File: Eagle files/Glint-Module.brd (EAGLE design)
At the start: 50.8 x 25.4 mm, 17 parts

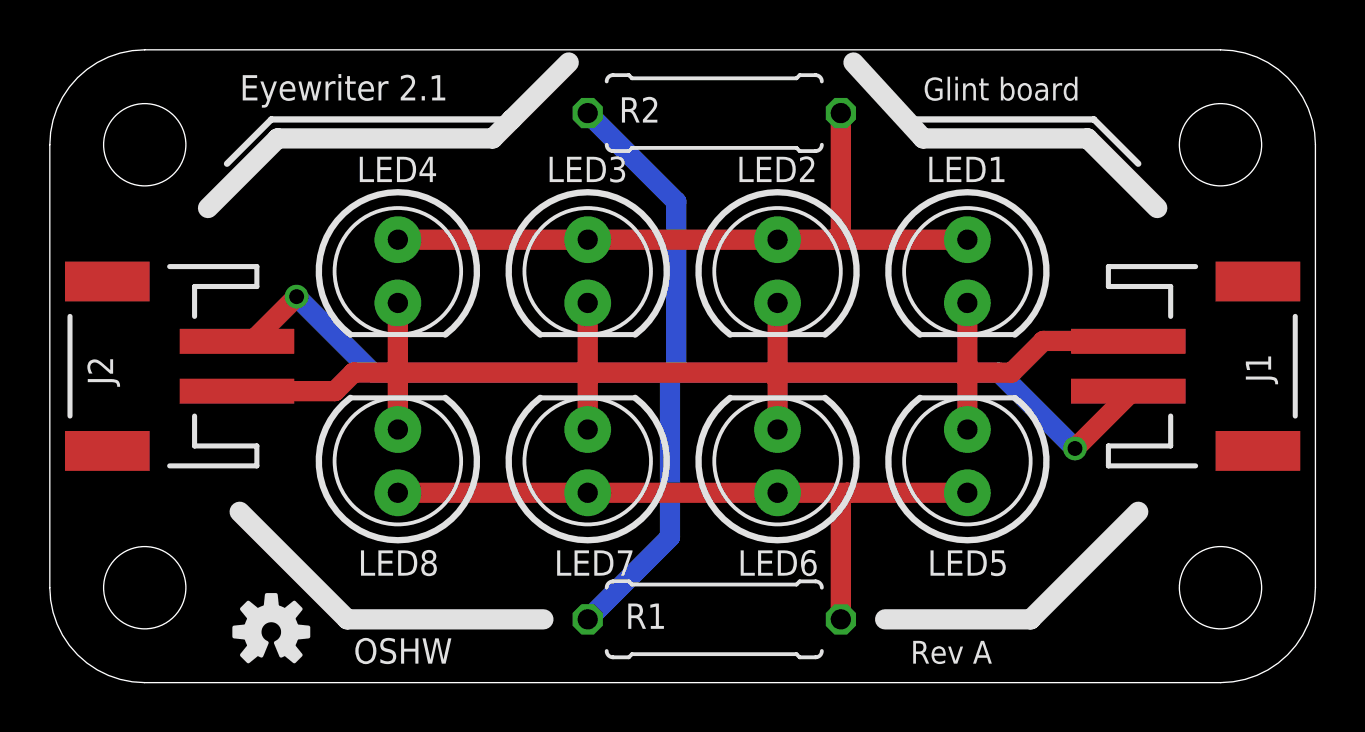
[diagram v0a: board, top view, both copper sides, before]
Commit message: Updated Eagle files + BOMs
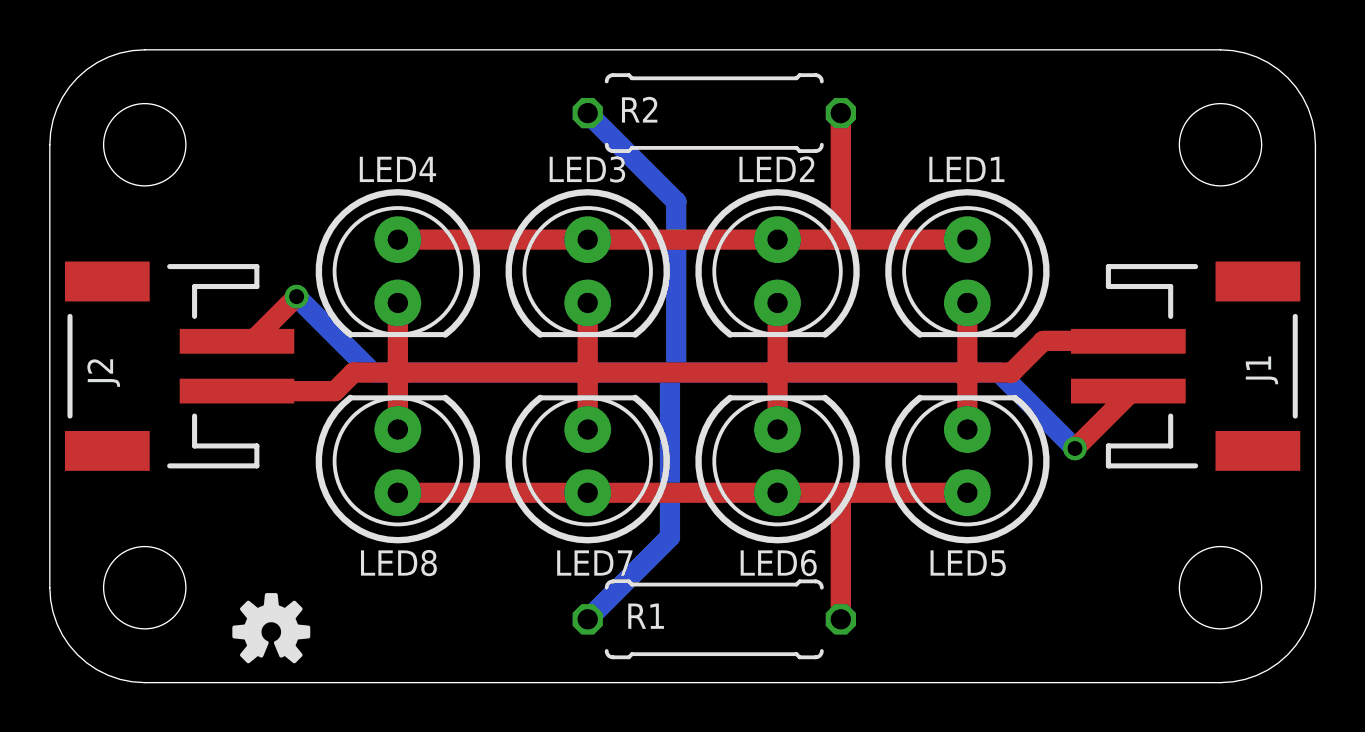
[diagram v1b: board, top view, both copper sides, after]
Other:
- board text added: "Designed by Jason Webb (http://jason-webb.info)"
- board text removed: "Designed by Jason Webb - http://jason-webb.info"
- board text removed: "Rev A"
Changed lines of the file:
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@@
 <layer number="20" name="Dimension" color="15" fill="1" visible="yes" active="yes"/>
 <layer number="21" name="tPlace" color="7" fill="1" visible="yes" active="yes"/>
-<layer number="22" name="bPlace" color="7" fill="1" visible="no" active="yes"/>
+<layer number="22" name="bPlace" color="7" fill="1" visible="yes" active="yes"/>
 <layer number="23" name="tOrigins" color="15" fill="1" visible="yes" active="yes"/>
-<layer number="24" name="bOrigins" color="15" fill="1" visible="no" active="yes"/>
+<layer number="24" name="bOrigins" color="15" fill="1" visible="yes" active="yes"/>
 <layer number="25" name="tNames" color="7" fill="1" visible="yes" active="yes"/>
-<layer number="26" name="bNames" color="7" fill="1" visible="no" active="yes"/>
+<layer number="26" name="bNames" color="7" fill="1" visible="yes" active="yes"/>
 <layer number="27" name="tValues" color="7" fill="1" visible="yes" active="yes"/>
-<layer number="28" name="bValues" color="7" fill="1" visible="no" active="yes"/>
+<layer number="28" name="bValues" color="7" fill="1" visible="yes" active="yes"/>
 <layer number="29" name="tStop" color="7" fill="3" visible="no" active="yes"/>
 <layer number="30" name="bStop" color="7" fill="6" visible="no" active="yes"/>
@@
 <layer number="37" name="tTest" color="7" fill="1" visible="no" active="yes"/>
 <layer number="38" name="bTest" color="7" fill="1" visible="no" active="yes"/>
-<layer number="39" name="tKeepout" color="4" fill="11" visible="no" active="yes"/>
-<layer number="40" name="bKeepout" color="1" fill="11" visible="no" active="yes"/>
-<layer number="41" name="tRestrict" color="4" fill="10" visible="no" active="yes"/>
-<layer number="42" name="bRestrict" color="1" fill="10" visible="no" active="yes"/>
-<layer number="43" name="vRestrict" color="2" fill="10" visible="no" active="yes"/>
+<layer number="39" name="tKeepout" color="4" fill="11" visible="yes" active="yes"/>
+<layer number="40" name="bKeepout" color="1" fill="11" visible="yes" active="yes"/>
+<layer number="41" name="tRestrict" color="4" fill="10" visible="yes" active="yes"/>
+<layer number="42" name="bRestrict" color="1" fill="10" visible="yes" active="yes"/>
+<layer number="43" name="vRestrict" color="2" fill="10" visible="yes" active="yes"/>
 <layer number="44" name="Drills" color="7" fill="1" visible="no" active="yes"/>
 <layer number="45" name="Holes" color="7" fill="1" visible="no" active="yes"/>
 <layer number="46" name="Milling" color="3" fill="1" visible="no" active="yes"/>
 <layer number="47" name="Measures" color="7" fill="1" visible="no" active="yes"/>
-<layer number="48" name="Document" color="7" fill="1" visible="no" active="yes"/>
-<layer number="49" name="Reference" color="7" fill="1" visible="no" active="yes"/>
+<layer number="48" name="Document" color="7" fill="1" visible="yes" active="yes"/>
+<layer number="49" name="Reference" color="7" fill="1" visible="yes" active="yes"/>
 <layer number="50" name="dxf" color="7" fill="1" visible="no" active="no"/>
-<layer number="51" name="tDocu" color="7" fill="1" visible="no" active="yes"/>
+<layer number="51" name="tDocu" color="7" fill="1" visible="yes" active="yes"/>
 <layer number="52" name="bDocu" color="7" fill="1" visible="no" active="yes"/>
 <layer number="53" name="tGND_GNDA" color="7" fill="9" visible="no" active="no"/>
@@
 <layer number="144" name="Drill_legend" color="7" fill="1" visible="no" active="yes"/>
 <layer number="151" name="HeatSink" color="7" fill="1" visible="no" active="yes"/>
-<layer number="199" name="Contour" color="7" fill="1" visible="no" active="yes"/>
+<layer number="199" name="Contour" color="7" fill="1" visible="yes" active="yes"/>
 <layer number="200" name="200bmp" color="1" fill="10" visible="no" active="yes"/>
 <layer number="201" name="201bmp" color="2" fill="10" visible="no" active="yes"/>
@@
 <board>
 <plain>
-<text x="7.62" y="23.368" size="1.016" layer="21" font="vector" ratio="16">Eyewriter 2.1</text>
-<text x="35.052" y="23.368" size="0.9144" layer="21" font="vector" ratio="12">Glint board</text>
-<wire x1="17.78" y1="21.844" x2="18.542" y2="22.606" width="0.8128" layer="21"/>
-<wire x1="18.542" y1="22.606" x2="20.828" y2="24.892" width="0.8128" layer="21"/>
-<wire x1="35.052" y1="21.844" x2="32.258" y2="24.892" width="0.8128" layer="21"/>
-<wire x1="17.78" y1="21.844" x2="9.144" y2="21.844" width="0.8128" layer="21"/>
-<wire x1="9.144" y1="21.844" x2="6.35" y2="19.05" width="0.8128" layer="21"/>
-<wire x1="35.052" y1="21.844" x2="41.656" y2="21.844" width="0.8128" layer="21"/>
-<wire x1="41.656" y1="21.844" x2="44.45" y2="19.05" width="0.8128" layer="21"/>
-<wire x1="34.544" y1="22.606" x2="41.91" y2="22.606" width="0.254" layer="21"/>
-<wire x1="41.91" y1="22.606" x2="43.688" y2="20.828" width="0.254" layer="21"/>
-<wire x1="18.542" y1="22.606" x2="8.89" y2="22.606" width="0.254" layer="21"/>
-<wire x1="8.89" y1="22.606" x2="7.112" y2="20.828" width="0.254" layer="21"/>
-<wire x1="7.62" y1="6.858" x2="11.938" y2="2.54" width="0.8128" layer="21"/>
-<wire x1="11.938" y1="2.54" x2="19.812" y2="2.54" width="0.8128" layer="21"/>
-<wire x1="43.688" y1="6.858" x2="39.37" y2="2.54" width="0.8128" layer="21"/>
-<wire x1="39.37" y1="2.54" x2="33.528" y2="2.54" width="0.8128" layer="21"/>
-<text x="12.192" y="0.762" size="1.016" layer="21" font="vector" ratio="16">OSHW</text>
-<text x="25.4" y="4.572" size="0.889" layer="22" font="vector" ratio="10" rot="MR0" align="center">Designed by Jason Webb - http://jason-webb.info</text>
-<text x="42.164" y="12.192" size="1.27" layer="22" font="vector" ratio="16" rot="MR0">Eyewrtier 2.1</text>
-<text x="21.082" y="12.446" size="1.27" layer="22" font="vector" ratio="16" rot="MR0">Glint board</text>
+<text x="7.62" y="23.368" size="1.016" layer="51" font="vector" ratio="16">Eyewriter 2.1</text>
+<text x="35.052" y="23.368" size="0.9144" layer="51" font="vector" ratio="12">Glint board</text>
+<wire x1="17.78" y1="21.844" x2="18.542" y2="22.606" width="0.8128" layer="51"/>
+<wire x1="18.542" y1="22.606" x2="20.828" y2="24.892" width="0.8128" layer="51"/>
+<wire x1="35.052" y1="21.844" x2="32.258" y2="24.892" width="0.8128" layer="51"/>
+<wire x1="17.78" y1="21.844" x2="9.144" y2="21.844" width="0.8128" layer="51"/>
+<wire x1="9.144" y1="21.844" x2="6.35" y2="19.05" width="0.8128" layer="51"/>
+<wire x1="35.052" y1="21.844" x2="41.656" y2="21.844" width="0.8128" layer="51"/>
+<wire x1="41.656" y1="21.844" x2="44.45" y2="19.05" width="0.8128" layer="51"/>
+<wire x1="34.544" y1="22.606" x2="41.91" y2="22.606" width="0.254" layer="51"/>
+<wire x1="41.91" y1="22.606" x2="43.688" y2="20.828" width="0.254" layer="51"/>
+<wire x1="18.542" y1="22.606" x2="8.89" y2="22.606" width="0.254" layer="51"/>
+<wire x1="8.89" y1="22.606" x2="7.112" y2="20.828" width="0.254" layer="51"/>
+<wire x1="7.62" y1="6.858" x2="11.938" y2="2.54" width="0.8128" layer="51"/>
+<wire x1="11.938" y1="2.54" x2="19.812" y2="2.54" width="0.8128" layer="51"/>
+<wire x1="43.688" y1="6.858" x2="39.37" y2="2.54" width="0.8128" layer="51"/>
+<wire x1="39.37" y1="2.54" x2="33.528" y2="2.54" width="0.8128" layer="51"/>
+<text x="12.192" y="0.762" size="1.016" layer="51" font="vector" ratio="16">OSHW</text>
+<text x="43.18" y="4.064" size="0.889" layer="52" font="vector" ratio="10" rot="MR0">Designed by Jason Webb (http://jason-webb.info)</text>
+<text x="42.164" y="12.192" size="1.27" layer="52" font="vector" ratio="16" rot="MR0">Eyewrtier 2.1</text>
+<text x="21.082" y="12.446" size="1.27" layer="52" font="vector" ratio="16" rot="MR0">Glint board</text>
 <wire x1="3.81" y1="0" x2="46.99" y2="0" width="0" layer="20"/>
 <wire x1="46.99" y1="0" x2="50.8" y2="3.81" width="0" layer="20" curve="90"/>
@@
 <wire x1="0" y1="21.59" x2="0" y2="3.81" width="0" layer="20"/>
 <wire x1="0" y1="3.81" x2="3.81" y2="0" width="0" layer="20" curve="90"/>
-<text x="34.544" y="0.762" size="0.9144" layer="21" font="vector" ratio="12">Rev A</text>
 </plain>
 <attributes>

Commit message: Updated Eagle files, including Gerbers and custom library
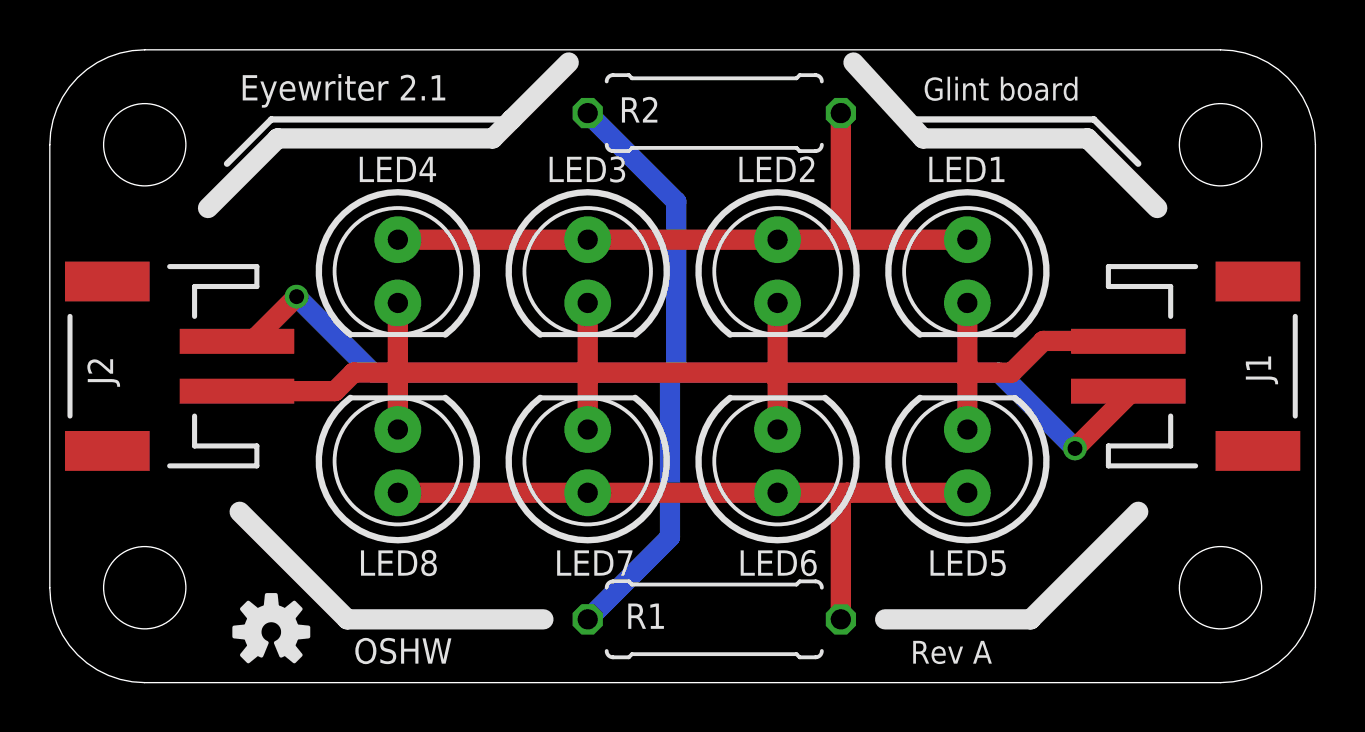
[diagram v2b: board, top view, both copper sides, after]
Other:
- board text added: "Designed by Jason Webb - http://jason-webb.info"
- board text added: "Rev A"
- board text removed: "Designed by Jason Webb (http://jason-webb.info)"
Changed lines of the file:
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@@
 <layer number="20" name="Dimension" color="15" fill="1" visible="yes" active="yes"/>
 <layer number="21" name="tPlace" color="7" fill="1" visible="yes" active="yes"/>
-<layer number="22" name="bPlace" color="7" fill="1" visible="yes" active="yes"/>
+<layer number="22" name="bPlace" color="7" fill="1" visible="no" active="yes"/>
 <layer number="23" name="tOrigins" color="15" fill="1" visible="yes" active="yes"/>
-<layer number="24" name="bOrigins" color="15" fill="1" visible="yes" active="yes"/>
+<layer number="24" name="bOrigins" color="15" fill="1" visible="no" active="yes"/>
 <layer number="25" name="tNames" color="7" fill="1" visible="yes" active="yes"/>
-<layer number="26" name="bNames" color="7" fill="1" visible="yes" active="yes"/>
+<layer number="26" name="bNames" color="7" fill="1" visible="no" active="yes"/>
 <layer number="27" name="tValues" color="7" fill="1" visible="yes" active="yes"/>
-<layer number="28" name="bValues" color="7" fill="1" visible="yes" active="yes"/>
+<layer number="28" name="bValues" color="7" fill="1" visible="no" active="yes"/>
 <layer number="29" name="tStop" color="7" fill="3" visible="no" active="yes"/>
 <layer number="30" name="bStop" color="7" fill="6" visible="no" active="yes"/>
@@
 <layer number="37" name="tTest" color="7" fill="1" visible="no" active="yes"/>
 <layer number="38" name="bTest" color="7" fill="1" visible="no" active="yes"/>
-<layer number="39" name="tKeepout" color="4" fill="11" visible="yes" active="yes"/>
-<layer number="40" name="bKeepout" color="1" fill="11" visible="yes" active="yes"/>
-<layer number="41" name="tRestrict" color="4" fill="10" visible="yes" active="yes"/>
-<layer number="42" name="bRestrict" color="1" fill="10" visible="yes" active="yes"/>
-<layer number="43" name="vRestrict" color="2" fill="10" visible="yes" active="yes"/>
+<layer number="39" name="tKeepout" color="4" fill="11" visible="no" active="yes"/>
+<layer number="40" name="bKeepout" color="1" fill="11" visible="no" active="yes"/>
+<layer number="41" name="tRestrict" color="4" fill="10" visible="no" active="yes"/>
+<layer number="42" name="bRestrict" color="1" fill="10" visible="no" active="yes"/>
+<layer number="43" name="vRestrict" color="2" fill="10" visible="no" active="yes"/>
 <layer number="44" name="Drills" color="7" fill="1" visible="no" active="yes"/>
 <layer number="45" name="Holes" color="7" fill="1" visible="no" active="yes"/>
 <layer number="46" name="Milling" color="3" fill="1" visible="no" active="yes"/>
 <layer number="47" name="Measures" color="7" fill="1" visible="no" active="yes"/>
-<layer number="48" name="Document" color="7" fill="1" visible="yes" active="yes"/>
-<layer number="49" name="Reference" color="7" fill="1" visible="yes" active="yes"/>
+<layer number="48" name="Document" color="7" fill="1" visible="no" active="yes"/>
+<layer number="49" name="Reference" color="7" fill="1" visible="no" active="yes"/>
 <layer number="50" name="dxf" color="7" fill="1" visible="no" active="no"/>
-<layer number="51" name="tDocu" color="7" fill="1" visible="yes" active="yes"/>
+<layer number="51" name="tDocu" color="7" fill="1" visible="no" active="yes"/>
 <layer number="52" name="bDocu" color="7" fill="1" visible="no" active="yes"/>
 <layer number="53" name="tGND_GNDA" color="7" fill="9" visible="no" active="no"/>
@@
 <layer number="144" name="Drill_legend" color="7" fill="1" visible="no" active="yes"/>
 <layer number="151" name="HeatSink" color="7" fill="1" visible="no" active="yes"/>
-<layer number="199" name="Contour" color="7" fill="1" visible="yes" active="yes"/>
+<layer number="199" name="Contour" color="7" fill="1" visible="no" active="yes"/>
 <layer number="200" name="200bmp" color="1" fill="10" visible="no" active="yes"/>
 <layer number="201" name="201bmp" color="2" fill="10" visible="no" active="yes"/>
@@
 <board>
 <plain>
-<text x="7.62" y="23.368" size="1.016" layer="51" font="vector" ratio="16">Eyewriter 2.1</text>
-<text x="35.052" y="23.368" size="0.9144" layer="51" font="vector" ratio="12">Glint board</text>
-<wire x1="17.78" y1="21.844" x2="18.542" y2="22.606" width="0.8128" layer="51"/>
-<wire x1="18.542" y1="22.606" x2="20.828" y2="24.892" width="0.8128" layer="51"/>
-<wire x1="35.052" y1="21.844" x2="32.258" y2="24.892" width="0.8128" layer="51"/>
-<wire x1="17.78" y1="21.844" x2="9.144" y2="21.844" width="0.8128" layer="51"/>
-<wire x1="9.144" y1="21.844" x2="6.35" y2="19.05" width="0.8128" layer="51"/>
-<wire x1="35.052" y1="21.844" x2="41.656" y2="21.844" width="0.8128" layer="51"/>
-<wire x1="41.656" y1="21.844" x2="44.45" y2="19.05" width="0.8128" layer="51"/>
-<wire x1="34.544" y1="22.606" x2="41.91" y2="22.606" width="0.254" layer="51"/>
-<wire x1="41.91" y1="22.606" x2="43.688" y2="20.828" width="0.254" layer="51"/>
-<wire x1="18.542" y1="22.606" x2="8.89" y2="22.606" width="0.254" layer="51"/>
-<wire x1="8.89" y1="22.606" x2="7.112" y2="20.828" width="0.254" layer="51"/>
-<wire x1="7.62" y1="6.858" x2="11.938" y2="2.54" width="0.8128" layer="51"/>
-<wire x1="11.938" y1="2.54" x2="19.812" y2="2.54" width="0.8128" layer="51"/>
-<wire x1="43.688" y1="6.858" x2="39.37" y2="2.54" width="0.8128" layer="51"/>
-<wire x1="39.37" y1="2.54" x2="33.528" y2="2.54" width="0.8128" layer="51"/>
-<text x="12.192" y="0.762" size="1.016" layer="51" font="vector" ratio="16">OSHW</text>
-<text x="43.18" y="4.064" size="0.889" layer="52" font="vector" ratio="10" rot="MR0">Designed by Jason Webb (http://jason-webb.info)</text>
-<text x="42.164" y="12.192" size="1.27" layer="52" font="vector" ratio="16" rot="MR0">Eyewrtier 2.1</text>
-<text x="21.082" y="12.446" size="1.27" layer="52" font="vector" ratio="16" rot="MR0">Glint board</text>
+<text x="7.62" y="23.368" size="1.016" layer="21" font="vector" ratio="16">Eyewriter 2.1</text>
+<text x="35.052" y="23.368" size="0.9144" layer="21" font="vector" ratio="12">Glint board</text>
+<wire x1="17.78" y1="21.844" x2="18.542" y2="22.606" width="0.8128" layer="21"/>
+<wire x1="18.542" y1="22.606" x2="20.828" y2="24.892" width="0.8128" layer="21"/>
+<wire x1="35.052" y1="21.844" x2="32.258" y2="24.892" width="0.8128" layer="21"/>
+<wire x1="17.78" y1="21.844" x2="9.144" y2="21.844" width="0.8128" layer="21"/>
+<wire x1="9.144" y1="21.844" x2="6.35" y2="19.05" width="0.8128" layer="21"/>
+<wire x1="35.052" y1="21.844" x2="41.656" y2="21.844" width="0.8128" layer="21"/>
+<wire x1="41.656" y1="21.844" x2="44.45" y2="19.05" width="0.8128" layer="21"/>
+<wire x1="34.544" y1="22.606" x2="41.91" y2="22.606" width="0.254" layer="21"/>
+<wire x1="41.91" y1="22.606" x2="43.688" y2="20.828" width="0.254" layer="21"/>
+<wire x1="18.542" y1="22.606" x2="8.89" y2="22.606" width="0.254" layer="21"/>
+<wire x1="8.89" y1="22.606" x2="7.112" y2="20.828" width="0.254" layer="21"/>
+<wire x1="7.62" y1="6.858" x2="11.938" y2="2.54" width="0.8128" layer="21"/>
+<wire x1="11.938" y1="2.54" x2="19.812" y2="2.54" width="0.8128" layer="21"/>
+<wire x1="43.688" y1="6.858" x2="39.37" y2="2.54" width="0.8128" layer="21"/>
+<wire x1="39.37" y1="2.54" x2="33.528" y2="2.54" width="0.8128" layer="21"/>
+<text x="12.192" y="0.762" size="1.016" layer="21" font="vector" ratio="16">OSHW</text>
+<text x="25.4" y="4.572" size="0.889" layer="22" font="vector" ratio="10" rot="MR0" align="center">Designed by Jason Webb - http://jason-webb.info</text>
+<text x="42.164" y="12.192" size="1.27" layer="22" font="vector" ratio="16" rot="MR0">Eyewrtier 2.1</text>
+<text x="21.082" y="12.446" size="1.27" layer="22" font="vector" ratio="16" rot="MR0">Glint board</text>
 <wire x1="3.81" y1="0" x2="46.99" y2="0" width="0" layer="20"/>
 <wire x1="46.99" y1="0" x2="50.8" y2="3.81" width="0" layer="20" curve="90"/>
@@
 <wire x1="0" y1="21.59" x2="0" y2="3.81" width="0" layer="20"/>
 <wire x1="0" y1="3.81" x2="3.81" y2="0" width="0" layer="20" curve="90"/>
+<text x="34.544" y="0.762" size="0.9144" layer="21" font="vector" ratio="12">Rev A</text>
 </plain>
 <attributes>
